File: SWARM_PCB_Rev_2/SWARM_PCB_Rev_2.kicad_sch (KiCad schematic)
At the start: 4 parts, among them J25 Conn_01x12_Pin, J26 Conn_01x12_Pin, J27 Conn_01x12_Pin, J28 Conn_01x13_Pin

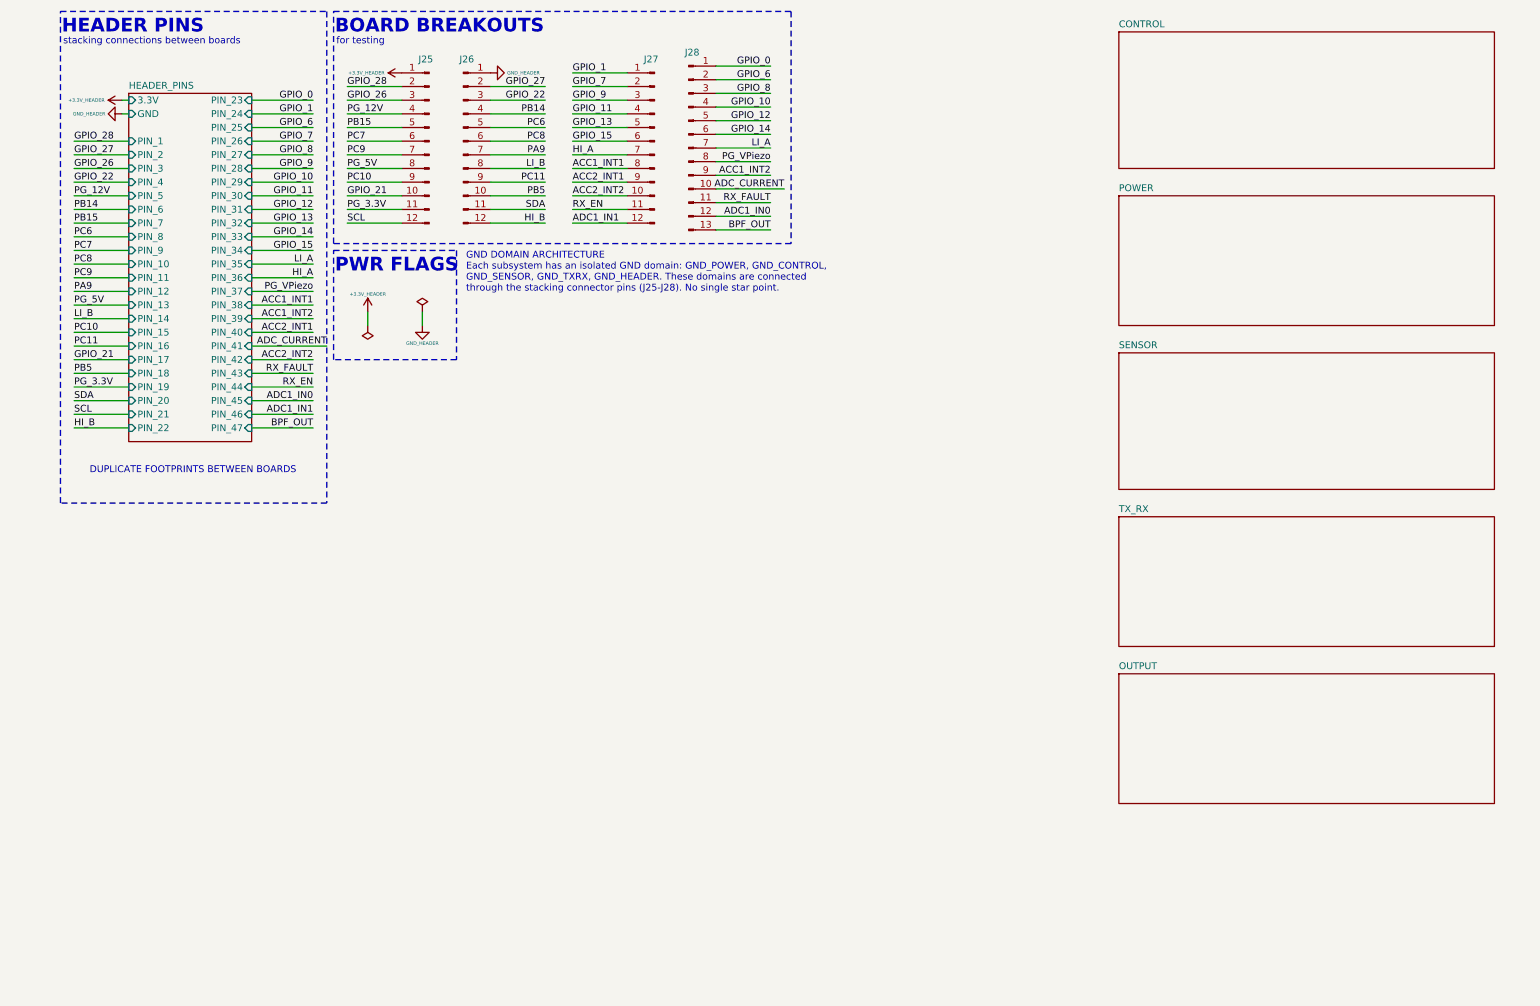
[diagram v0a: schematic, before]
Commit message: Cleaned up Schematic and Exported
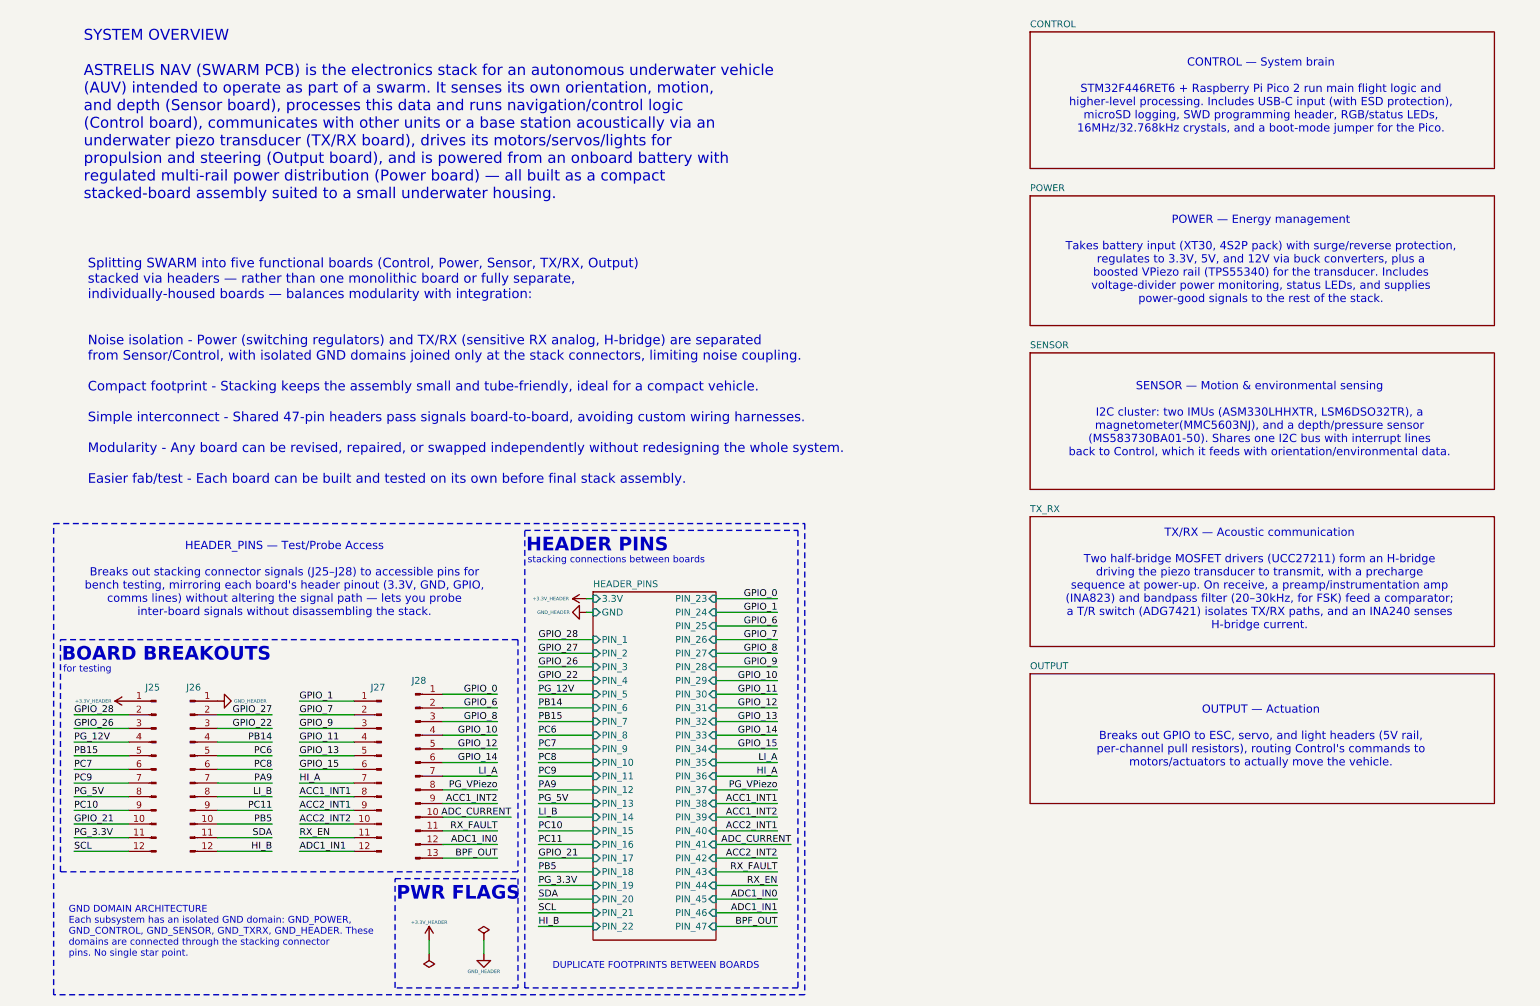
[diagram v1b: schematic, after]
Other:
- note added: "CONTROL — System brain STM32F446RET6 + Raspberry Pi Pico 2 run main flight logic and higher-level processing. Includes USB-C input (with ESD protection), microSD logging, SWD programming header, RGB/status LEDs, 16MHz/32.768kHz crystals, and a boot-mode jumper for the Pico."
- note added: "GND DOMAIN ARCHITECTURE Each subsystem has an isolated GND domain: GND_POWER, GND_CONTROL, GND_SENSOR, GND_TXRX, GND_HEADER. These domains are connected through the stacking connector pins. No single star point."
- note added: "HEADER_PINS — Test/Probe Access Breaks out stacking connector signals (J25–J28) to accessible pins for bench testing, mirroring each board's header pinout (3.3V, GND, GPIO, comms lines) without altering the signal path — lets you probe inter-board signals without disassembling the stack."
- note added: "OUTPUT — Actuation Breaks out GPIO to ESC, servo, and light headers (5V rail, per-channel pull resistors), routing Control's commands to motors/actuators to actually move the vehicle."
- note added: "POWER — Energy management Takes battery input (XT30, 4S2P pack) with surge/reverse protection, regulates to 3.3V, 5V, and 12V via buck converters, plus a boosted VPiezo rail (TPS55340) for the transducer. Includes voltage-divider power monitoring, status LEDs, and supplies power-good signals to the rest of the stack."
- note added: "SENSOR — Motion & environmental sensing I2C cluster: two IMUs (ASM330LHHXTR, LSM6DSO32TR), a magnetometer(MMC5603NJ), and a depth/pressure sensor (MS583730BA01-50). Shares one I2C bus with interrupt lines back to Control, which it feeds with orientation/environmental data."
- note added: "SYSTEM OVERVIEW ASTRELIS NAV (SWARM PCB) is the electronics stack for an autonomous underwater vehicle (AUV) intended to operate as part of a swarm. It senses its own orientation, motion, and depth (Sensor board), processes this data and runs navigation/control logic (Control board), communicates with other units or a base station acoustically via an underwater piezo transducer (TX/RX board), dri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"
- note added: "Splitting SWARM into five functional boards (Control, Power, Sensor, TX/RX, Output) stacked via headers — rather than one monolithic board or fully separate, individually-housed boards — balances modularity with integration: Noise isolation - Power (switching regulators) and TX/RX (sensitive RX analog, H-bridge) are separated from Sensor/Control, with isolated GND domains joined only at the stack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"
- note added: "TX/RX — Acoustic communication Two half-bridge MOSFET drivers (UCC27211) form an H-bridge driving the piezo transducer to transmit, with a precharge sequence at power-up. On receive, a preamp/instrumentation amp (INA823) and bandpass filter (20–30kHz, for FSK) feed a comparator; a T/R switch (ADG7421) isolates TX/RX paths, and an INA240 senses H-bridge current."
- note removed: "GND DOMAIN ARCHITECTURE Each subsystem has an isolated GND domain: GND_POWER, GND_CONTROL, GND_SENSOR, GND_TXRX, GND_HEADER. These domains are connected through the stacking connector pins (J25-J28). No single star point."
- moved on the sheet: J25, J26, J27, J28
